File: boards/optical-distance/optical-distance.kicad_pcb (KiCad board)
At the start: 2 copper layers, 23 x 19.5 mm, 7 parts, among them J1 CONN_02X03, M3 MountingHole_3.2mm_M3, U1 DS9638

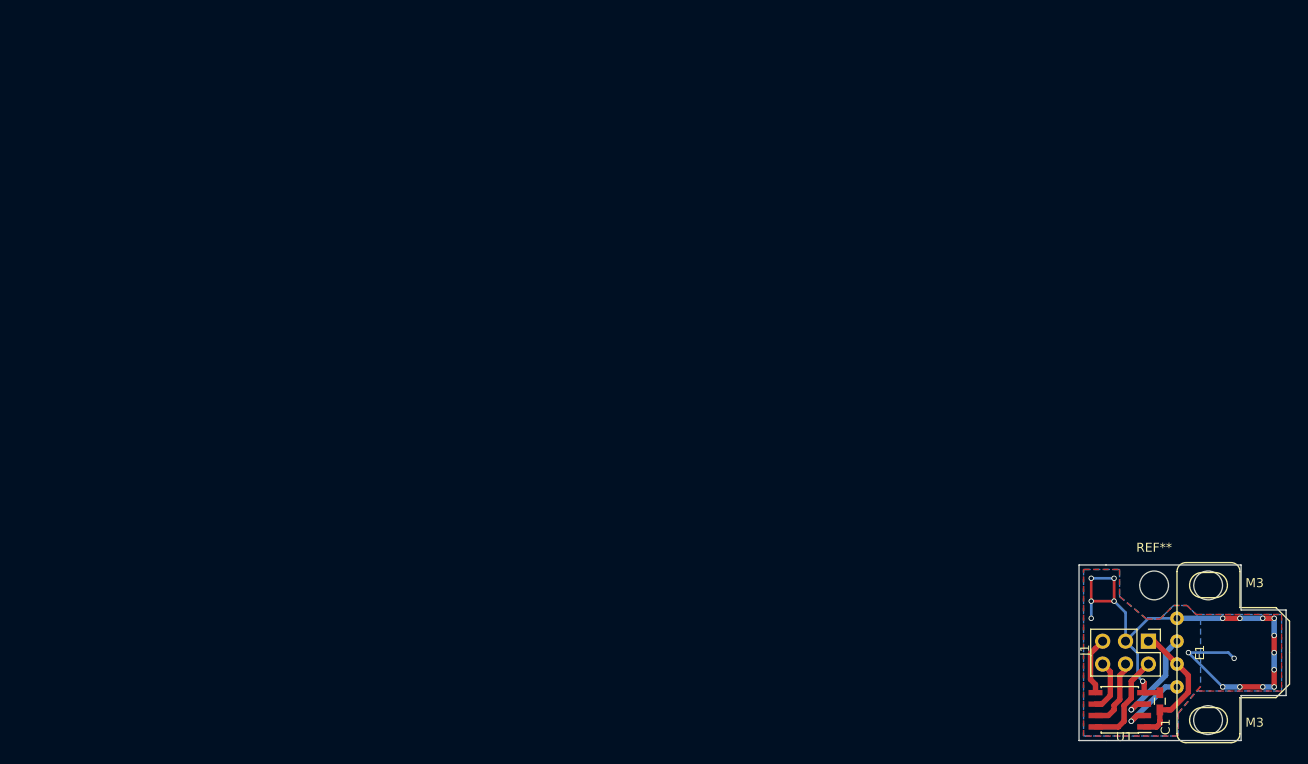
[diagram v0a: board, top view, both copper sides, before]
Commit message: [docs] export all board layouts
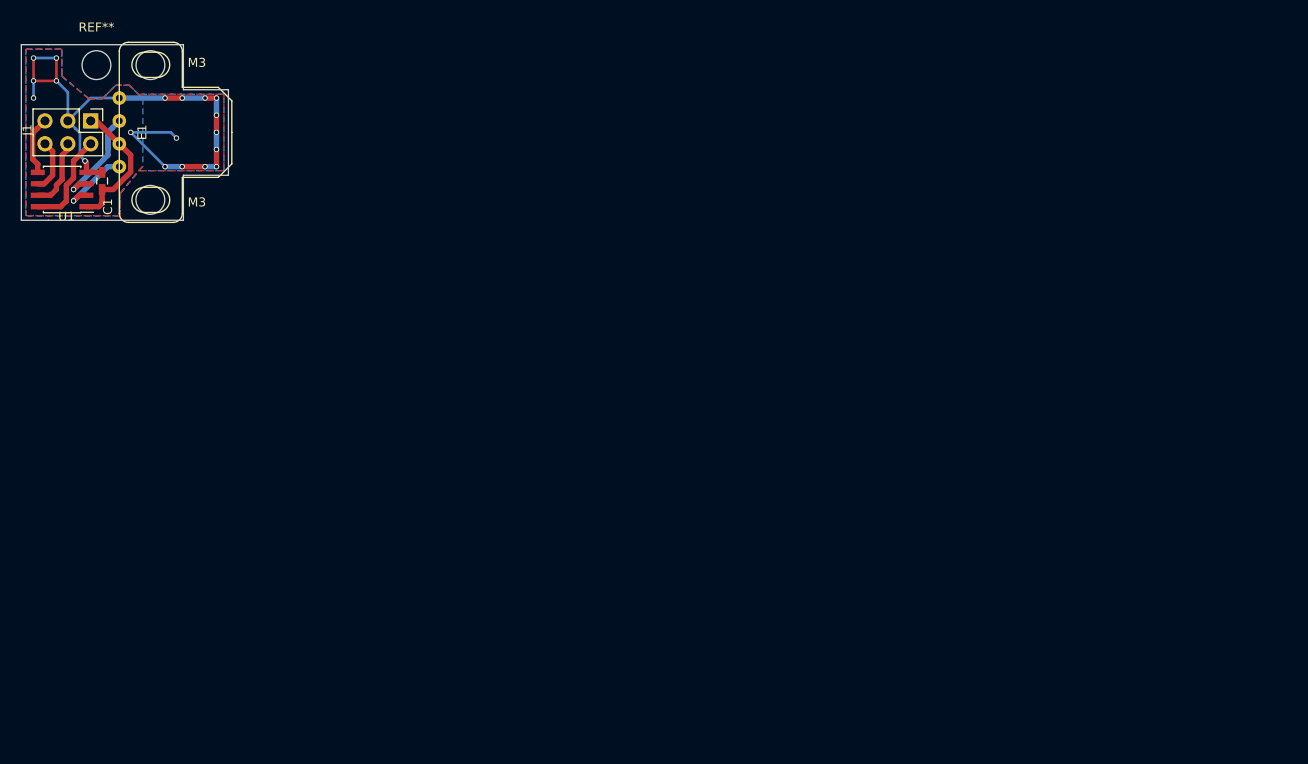
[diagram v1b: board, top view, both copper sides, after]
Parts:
- moved J1 130.9 mm to (62.2, 43.2)
- moved M3 130.9 mm to (68.9, 37.0)
- moved M3 130.9 mm to (68.9, 51.9)
- moved C1 130.9 mm to (63.5, 49.9)
- moved E1 130.9 mm to (65.4, 44.5)
- moved REF** 130.9 mm to (62.9, 37.0)
- moved U1 130.9 mm to (59.1, 50.8)
